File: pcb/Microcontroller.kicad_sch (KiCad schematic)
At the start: 39 parts, among them J1 PDI, SW2 START, SW3 STOP, U3 ATxmega16A4U-A, Y1 8MHz

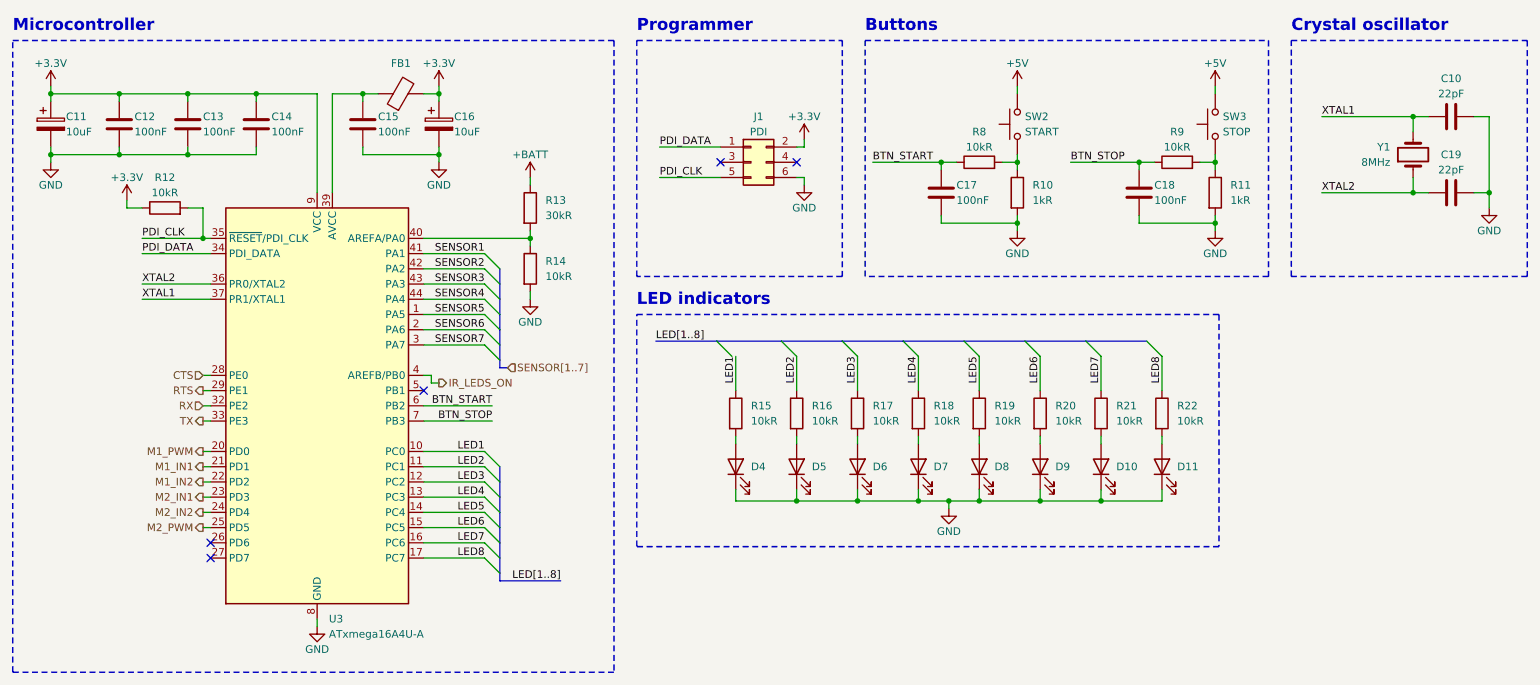
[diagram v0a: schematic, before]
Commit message: [pcb] Initial layout
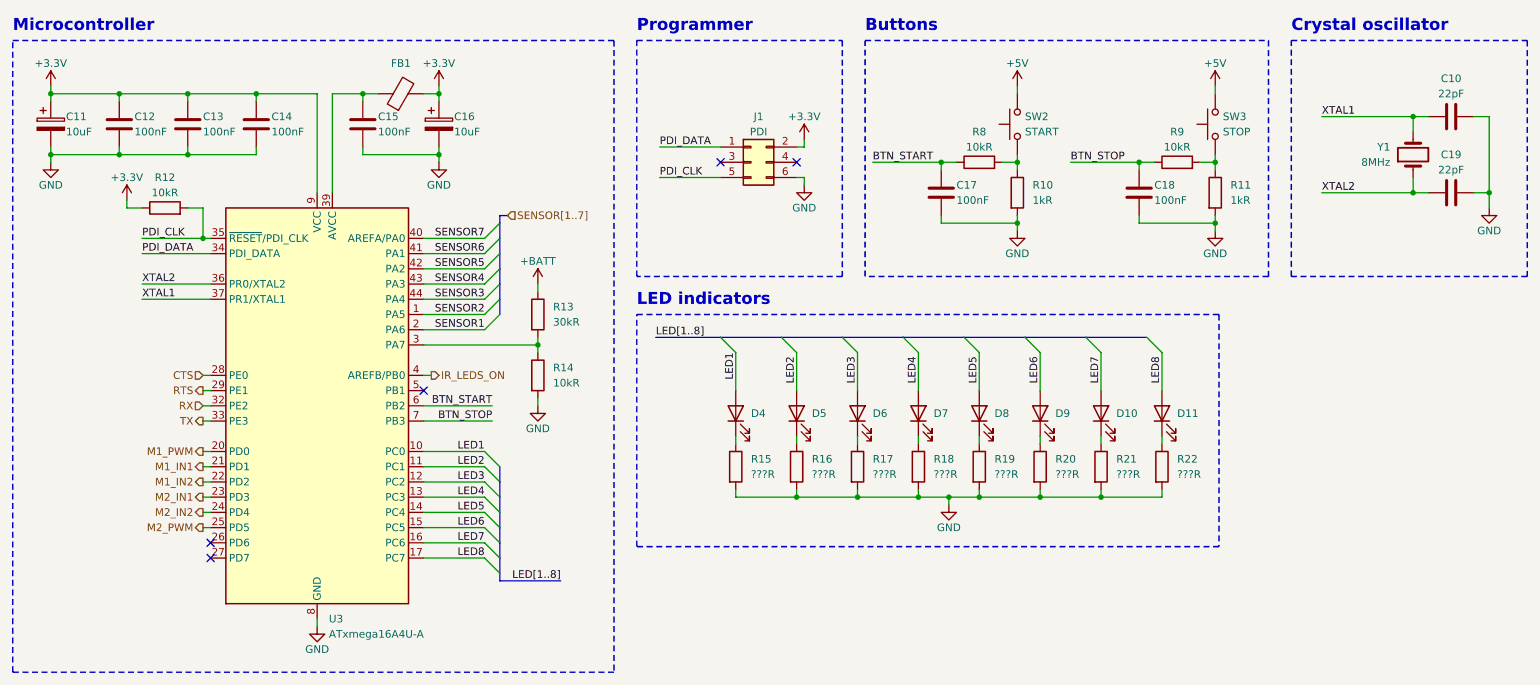
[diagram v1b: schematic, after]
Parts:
- R15, R16, R17, R18, R19, R20, R21, R22: value 10kR -> ???R
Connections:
- net GND: now also R15.2, R16.2, R17.2, R18.2, R19.2, R20.2, R21.2, R22.2; no longer D10.1 (K), D11.1 (K), D4.1 (K), D5.1 (K), D6.1 (K), D7.1 (K), D8.1 (K), D9.1 (K)
- net LED1: now also D4.2 (A); no longer R15.1
- net LED2: now also D5.2 (A); no longer R16.1
- net LED3: now also D6.2 (A); no longer R17.1
- net LED4: now also D7.2 (A); no longer R18.1
- net LED5: now also D8.2 (A); no longer R19.1
- net LED6: now also D9.2 (A); no longer R20.1
- net LED7: now also D10.2 (A); no longer R21.1
- net LED8: now also D11.2 (A); no longer R22.1
- net SENSOR1: now also U3.2 (PA6); no longer U3.41 (PA1)
- net SENSOR2: now also U3.1 (PA5); no longer U3.42 (PA2)
- net SENSOR3: now also U3.44 (PA4); no longer U3.43 (PA3)
- net SENSOR4: now also U3.43 (PA3); no longer U3.44 (PA4)
- net SENSOR5: now also U3.42 (PA2); no longer U3.1 (PA5)
- net SENSOR6: now also U3.41 (PA1); no longer U3.2 (PA6)
- net SENSOR7: now also U3.40 (AREFA/PA0); no longer U3.3 (PA7)
- net at R13.2, R14.1: now also U3.3 (PA7); no longer U3.40 (AREFA/PA0)
- new net: D4.1 (K), R15.1
- new net: D6.1 (K), R17.1
- new net: D7.1 (K), R18.1
- new net: D9.1 (K), R20.1
- new net: D11.1 (K), R22.1
- new net: D8.1 (K), R19.1
- new net: D10.1 (K), R21.1
- new net: D5.1 (K), R16.1
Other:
- moved on the sheet: D10, D11, D4, D5, D6, D7, D8, D9, R13, R14, R15, R16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
